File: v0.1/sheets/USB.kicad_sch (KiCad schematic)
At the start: 17 parts

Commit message: [HW] [PCB] v0.1_Y48 revision
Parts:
- D4: LCSC Part # (none) -> C1974707
- L6: LCSC Part # (none) -> C2651144
- Q2: LCSC Part # (none) -> C2965326
- TP7: now left out of the parts list
- U7: LCSC Part # (none) -> C2927037
- U8: LCSC Part # (none) -> C1121848
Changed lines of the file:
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@@
+			)
+		)
+		(property "LCSC Part #" "C2965326"
+			(at 173.99 29.21 90)
+			(effects
+				(font
+					(size 1.27 1.27)
+				)
+				(hide yes)
 			)
 		)
@@
 			)
 		)
+		(property "LCSC Part #" "C1974707"
+			(at 114.3 105.41 90)
+			(effects
+				(font
+					(size 1.27 1.27)
+				)
+				(hide yes)
+			)
+		)
 		(pin "2"
 		)
@@
 			)
 		)
+		(property "LCSC Part #" "C1121848"
+			(at 204.47 66.04 0)
+			(effects
+				(font
+					(size 1.27 1.27)
+				)
+				(hide yes)
+			)
+		)
 		(pin "3"
 		)
@@
 		(unit 1)
 		(exclude_from_sim no)
-		(in_bom yes)
+		(in_bom no)
 		(on_board yes)
 		(dnp no)
@@
 			)
 		)
+		(property "LCSC Part #" "C2927037"
+			(at 128.27 64.77 0)
+			(effects
+				(font
+					(size 1.27 1.27)
+				)
+				(hide yes)
+			)
+		)
 		(pin "4"
 		)
@@
 			(at 199.39 105.41 0)
 			(effects
+				(font
+					(size 1.27 1.27)
+				)
+				(hide yes)
+			)
+		)
+		(property "LCSC Part #" "C2651144"
+			(at 199.39 105.41 0)
+			(effects

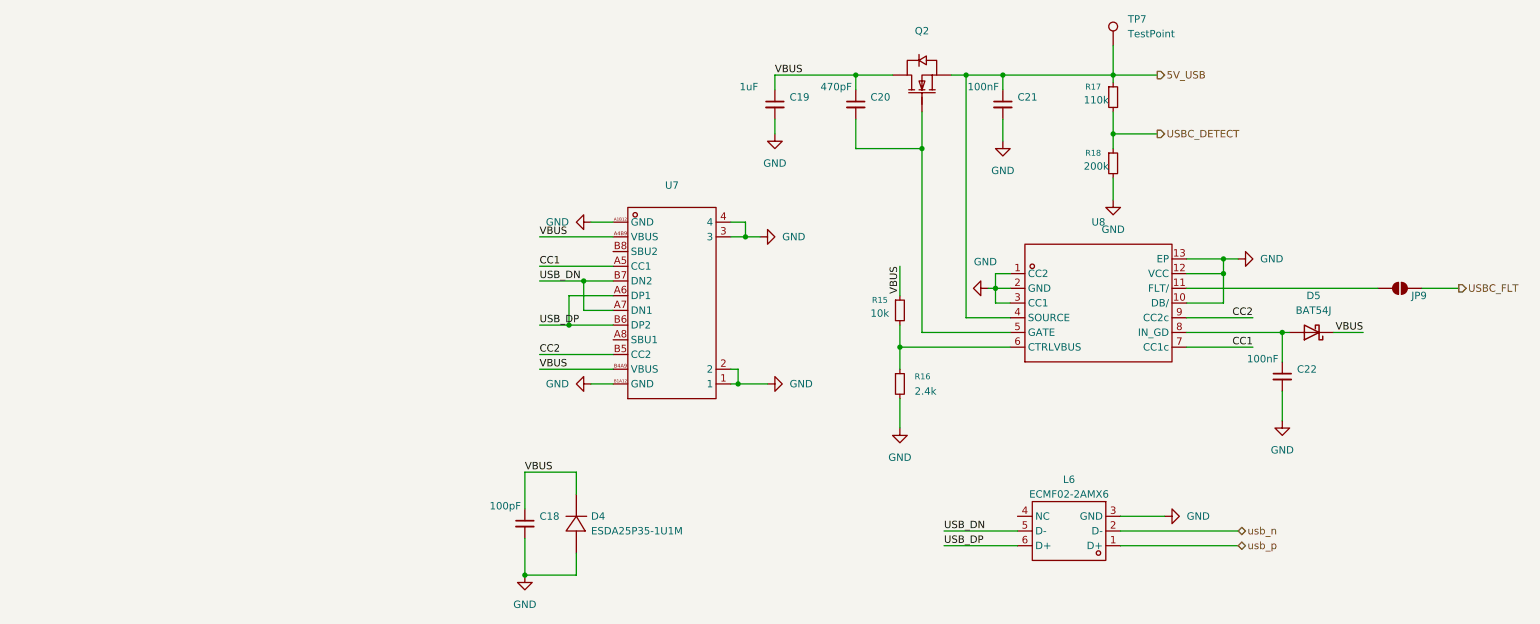
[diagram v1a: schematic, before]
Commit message: [HW] [PCB] revision v0.1_Y49
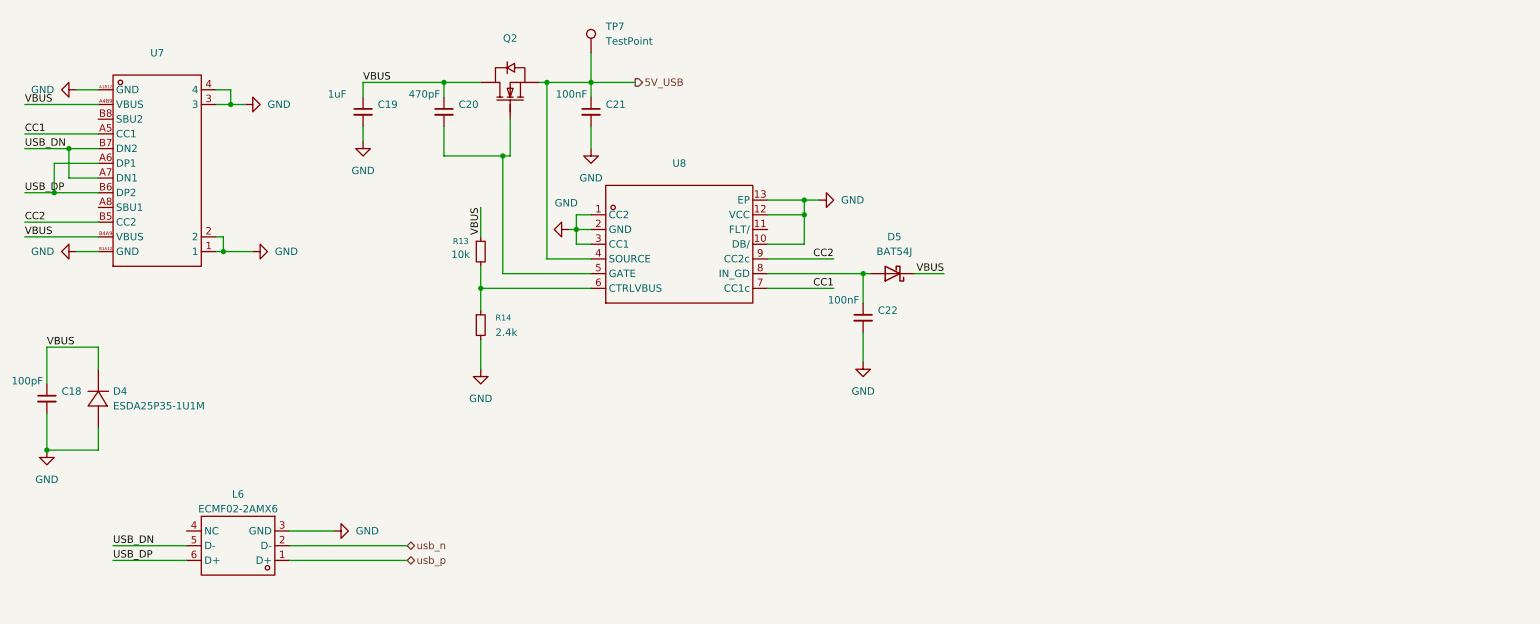
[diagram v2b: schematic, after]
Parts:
- removed JP9: SolderJumper_2_Open, Jumper:SolderJumper-2_P1.3mm_Open_TrianglePad1.0x1.5mm, symbol Jumper:SolderJumper_2_Open
- removed R17: 110k, Resistor_SMD:R_0603_1608Metric, symbol Device:R_Small
- removed R18: 200k, Resistor_SMD:R_0603_1608Metric, symbol Device:R_Small
- R13: renamed from R15; footprint Resistor_SMD:R_0603_1608Metric -> Resistor_SMD:R_0402_1005Metric
- R14: renamed from R16; footprint Resistor_SMD:R_0603_1608Metric -> Resistor_SMD:R_0402_1005Metric
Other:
- moved on the sheet: C18, C19, C20, C21, C22, D4, D5, L6, Q2, R13, R14, TP7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
